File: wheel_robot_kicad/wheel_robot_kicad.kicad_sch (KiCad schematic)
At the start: 7 parts, among them M1 Motor_DC, M2 Motor_DC, U1 ESP32-C6-MINI-1, U2 LM2596S-3.3, U3 BMI160, U4 DRV8833PW, U5 DRV8833PW

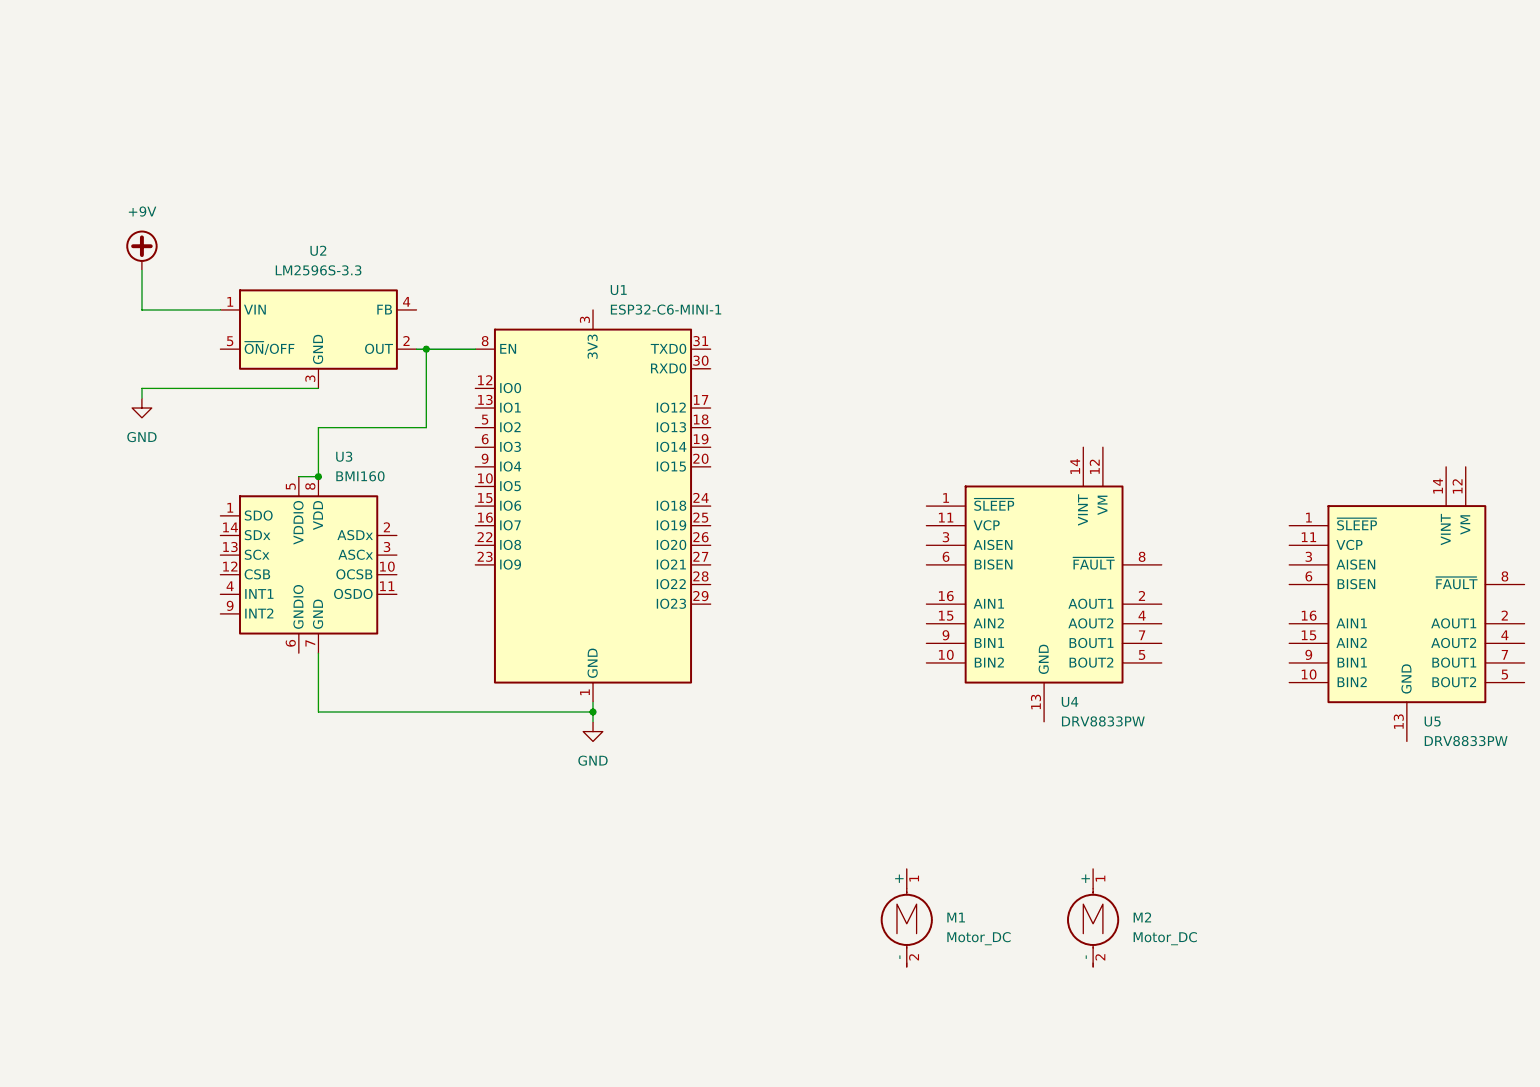
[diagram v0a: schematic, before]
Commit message: added additional IMU documentation
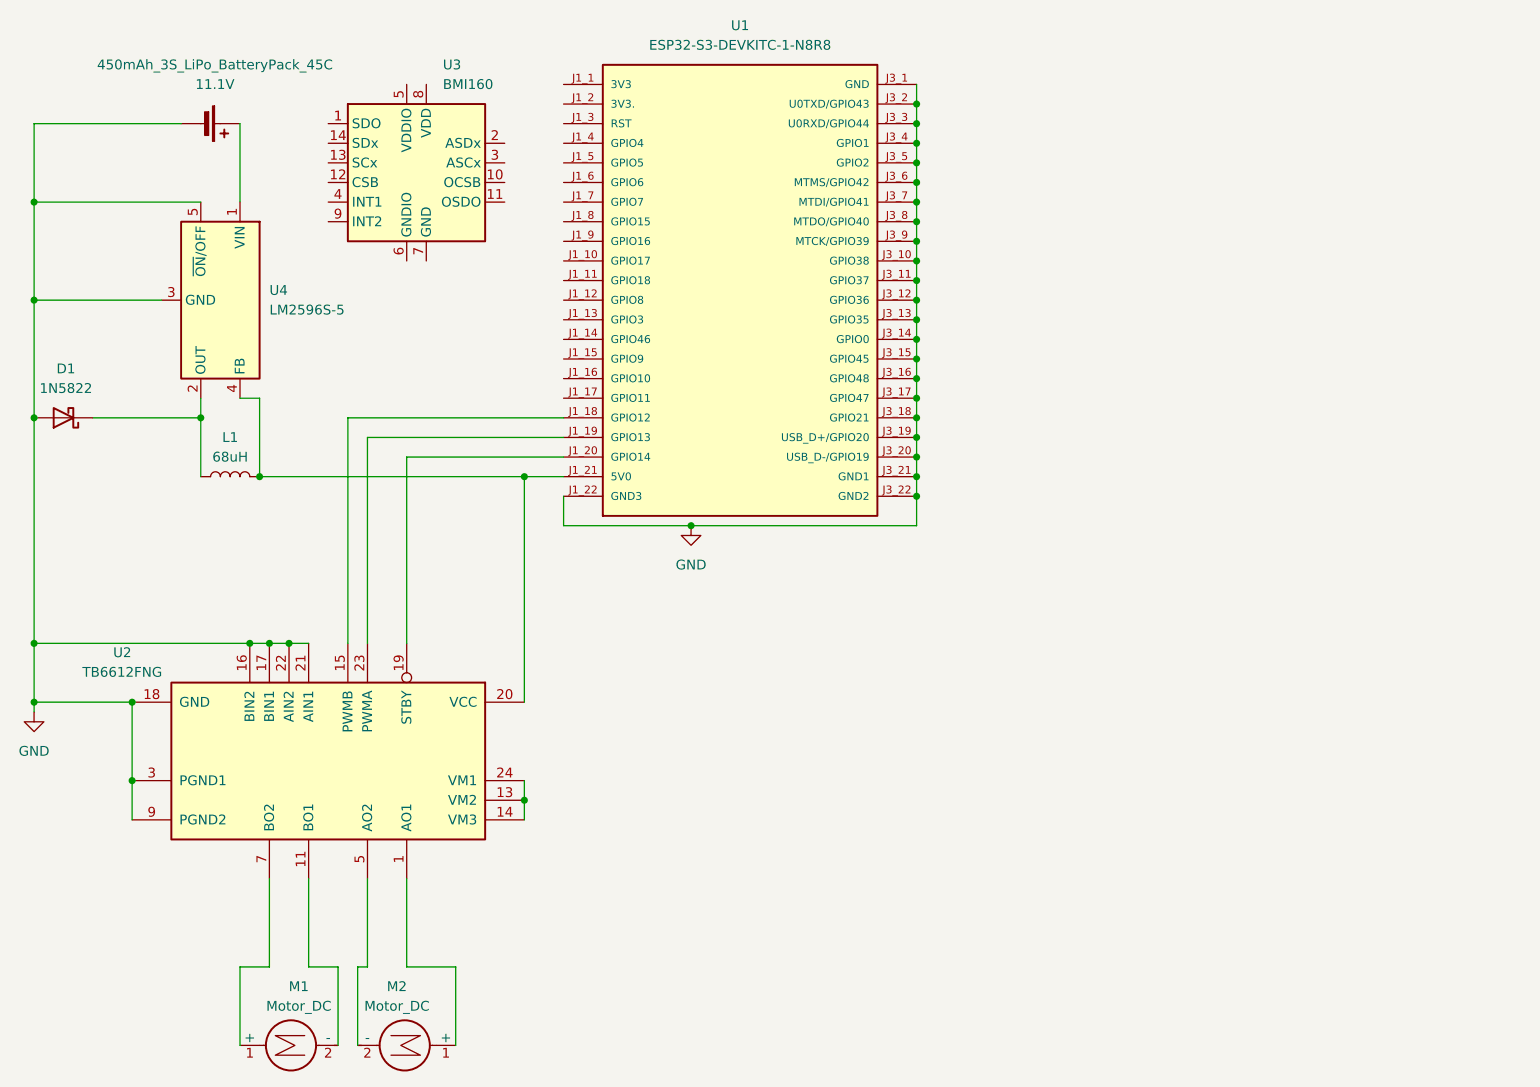
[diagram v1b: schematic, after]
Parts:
- removed U1: ESP32-C6-MINI-1, RF_Module:ESP32-C6-MINI-1, symbol RF_Module:ESP32-C6-MINI-1
- removed U2: LM2596S-3.3, Package_TO_SOT_SMD:TO-263-5_TabPin3, symbol Regulator_Switching:LM2596S-3.3
- removed U4, U5: DRV8833PW, Package_SO:TSSOP-16_4.4x5mm_P0.65mm, symbol Driver_Motor:DRV8833PW
- added 450mAh_3S_LiPo_BatteryPack_45C: 11.1V, symbol Device:Battery_Cell
- added D1: 1N5822, Diode_THT:D_DO-201AD_P15.24mm_Horizontal, symbol Diode:1N5822
- added L1: 68uH, symbol Device:L
- added U1: ESP32-S3-DEVKITC-1-N8R8, ESP32-S3-DEVKITC-1-N8R8:ESP32-S3-DEVKITC-1-N8R8, symbol ESP32-S3-DEVKITC-1-N8R8:ESP32-S3-DEVKITC-1-N8R8
- added U2: TB6612FNG, Package_SO:SSOP-24_5.3x8.2mm_P0.65mm, symbol Driver_Motor:TB6612FNG
- added U4: LM2596S-5, Package_TO_SOT_SMD:TO-263-5_TabPin3, symbol Regulator_Switching:LM2596S-5
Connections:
- net GND: now also 450mAh_3S_LiPo_BatteryPack_45C.2 (-), D1.2 (A), U1.J1_22 (GND3), U1.J3_1 (GND), U1.J3_10 (GPIO38), U1.J3_11 (GPIO37), U1.J3_12 (GPIO36), U1.J3_13 (GPIO35), U1.J3_14 (GPIO0), U1.J3_15 (GPIO45), U1.J3_16 (GPIO48), U1.J3_17 (GPIO47), U1.J3_18 (GPIO21), U1.J3_19 (USB_D+/GPIO20), U1.J3_2 (U0TXD/GPIO43), U1.J3_20 (USB_D-/GPIO19), U1.J3_21 (GND1), U1.J3_22 (GND2), U1.J3_3 (U0RXD/GPIO44), U1.J3_4 (GPIO1), U1.J3_5 (GPIO2), U1.J3_6 (MTMS/GPIO42), U1.J3_7 (MTDI/GPIO41), U1.J3_8 (MTDO/GPIO40), U1.J3_9 (MTCK/GPIO39), U2.10 (PGND2), U2.16 (BIN2), U2.17 (BIN1), U2.18 (GND), U2.21 (AIN1), U2.22 (AIN2), U2.3 (PGND1), U2.4 (PGND1), U2.9 (PGND2), U4.3 (GND), U4.5 (~{ON}/OFF); no longer U3.7 (GND)
- net at U3.5 (VDDIO): no longer U3.8 (VDD)
- net at M1.1 (+): now also U2.7 (BO2), U2.8 (BO2)
- net at M1.2 (-): now also U2.11 (BO1), U2.12 (BO1)
- net at M2.1 (+): now also U2.1 (AO1), U2.2 (AO1)
- net at M2.2 (-): now also U2.5 (AO2), U2.6 (AO2)
- new net: D1.1 (K), L1.1, U4.2 (OUT)
- new net: 450mAh_3S_LiPo_BatteryPack_45C.1 (+), U4.1 (VIN)
- new net: U1.J1_18 (GPIO12), U2.15 (PWMB)
- new net: U1.J1_19 (GPIO13), U2.23 (PWMA)
- new net: U1.J1_20 (GPIO14), U2.19 (STBY)
- new net: L1.2, U1.J1_21 (5V0), U2.20 (VCC), U4.4 (FB)
- new net: U2.13 (VM2), U2.14 (VM3), U2.24 (VM1)
